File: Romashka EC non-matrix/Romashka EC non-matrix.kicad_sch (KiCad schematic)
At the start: 39 parts, among them J1 Daisy40, J2 RS40, J3 JJ40, J4 JSB USB, J5 SOICbite, U1 STM32G474CBTx, U2 USBLC6-2P6, U3 TPS7A2033, Y1 Crystal_GND24_Small

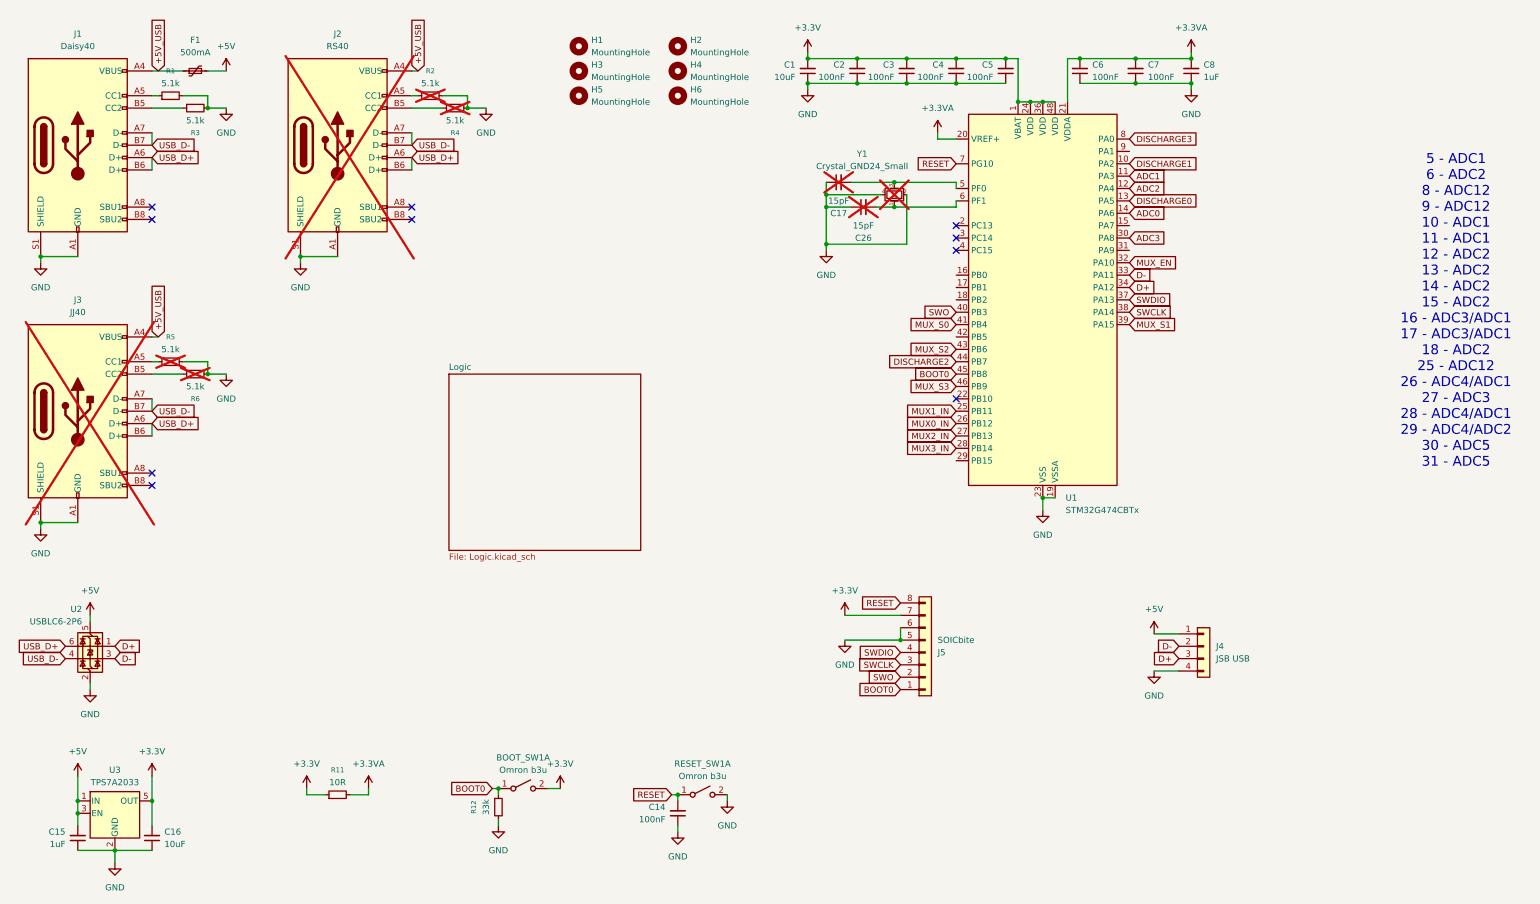
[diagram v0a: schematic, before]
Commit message: 23.08.2026
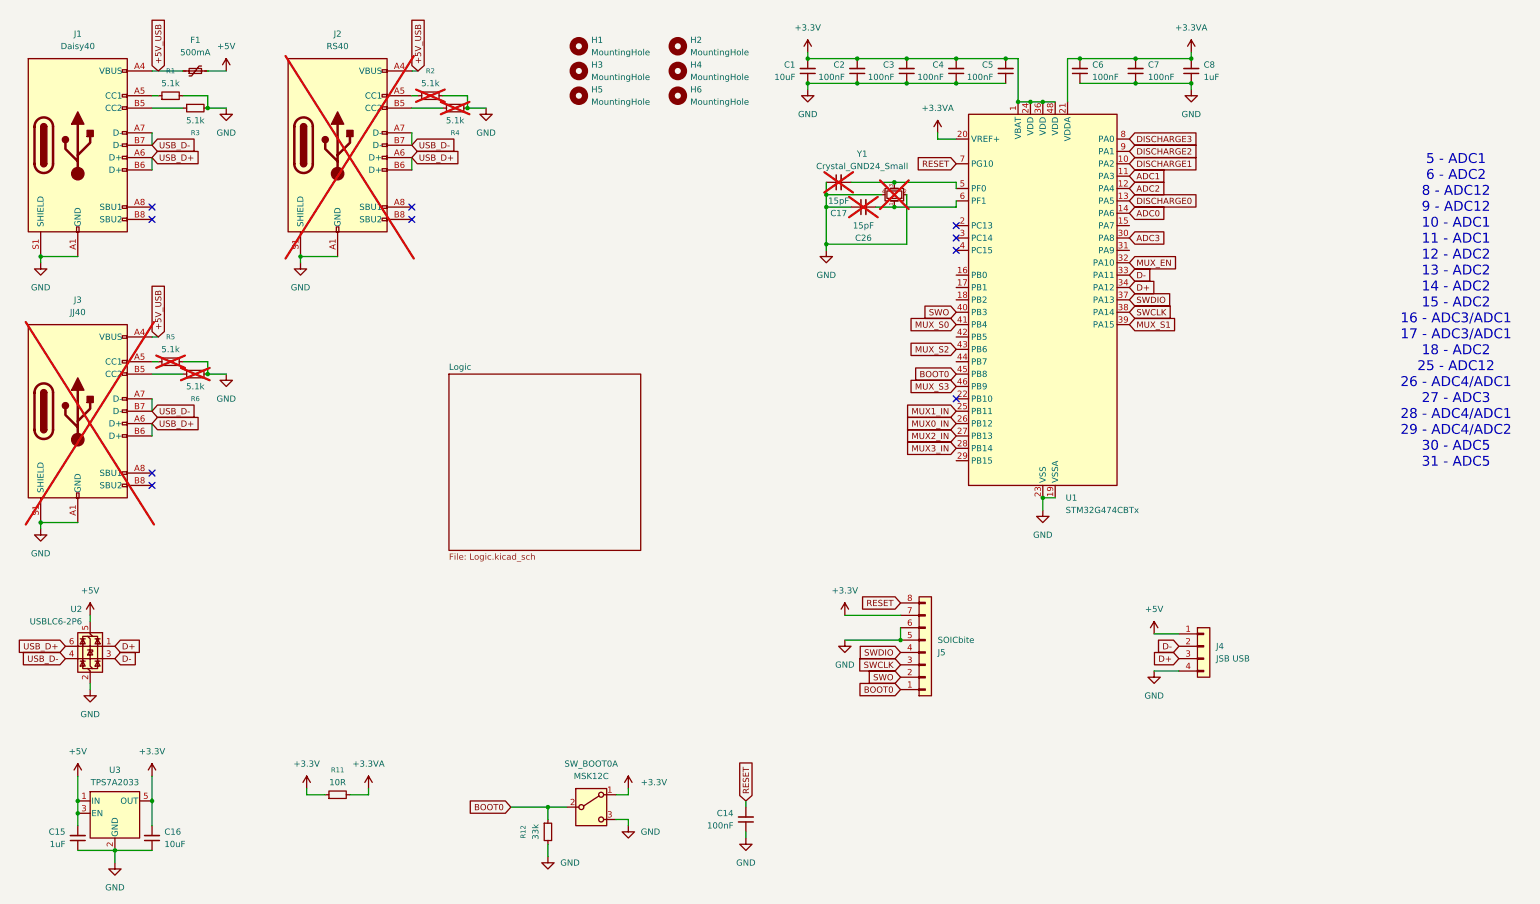
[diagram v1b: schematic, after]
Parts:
- removed BOOT_SW1, RESET_SW1: Omron b3u, Button_Switch_SMD:SW_SPST_B3U-1000P, symbol Switch:SW_DPST_x2
- added SW_BOOT0: MSK12C, FriedSoul_switches:slider-msk12c, symbol Switch:SW_DPDT_x2
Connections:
- net +3.3V: now also SW_BOOT0.1 (A)
- net BOOT0: now also SW_BOOT0.2 (B)
- net DISCHARGE2: now also U1.9 (PA1); no longer U1.44 (PB7)
- net GND: now also SW_BOOT0.3 (C)
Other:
- moved on the sheet: C14, R12
